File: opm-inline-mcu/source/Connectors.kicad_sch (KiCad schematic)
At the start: 32 parts, among them J1 Info, J2 VCC_IO, J3 PWMx6, J4 Fan, J6 Current Sensing, Q7 WSD90P06DN56, U2 TerminalBlock_2_P5.08mm, U3 TerminalBlock_3_P5.08mm

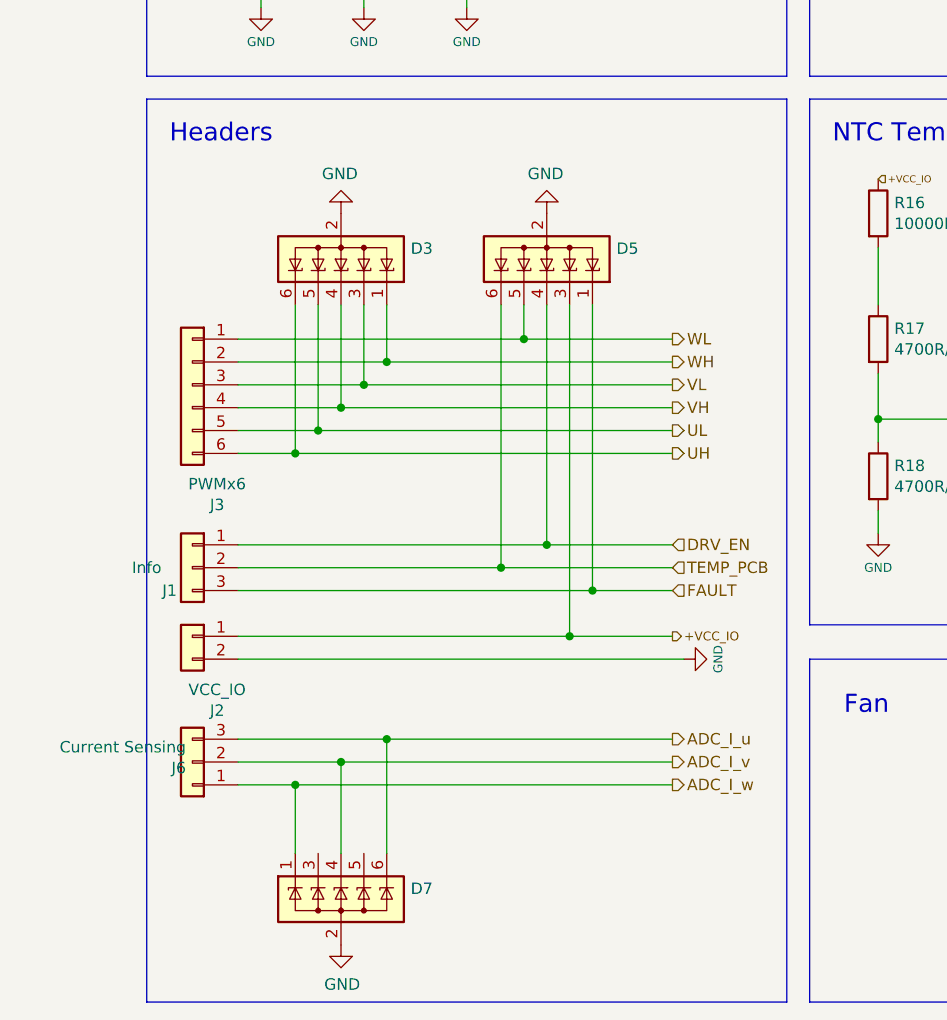
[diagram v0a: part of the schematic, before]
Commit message: update mcu
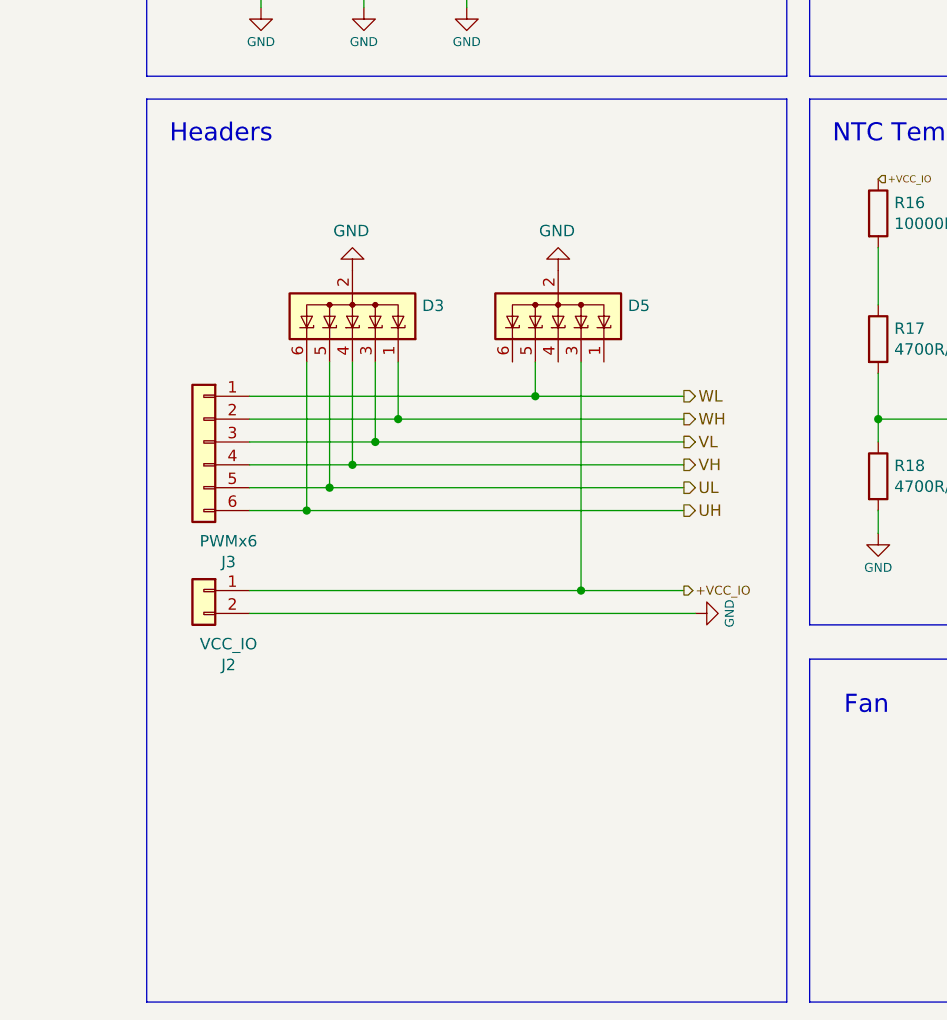
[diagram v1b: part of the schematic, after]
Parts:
- removed D7: NUP4114UCW1T2G, Libraries:NUP4114UCW1T2G, symbol Power_Protection:SP0505BAJT
- removed J1: Info, Connector_JST:JST_PH_B3B-PH-K_1x03_P2.00mm_Vertical, symbol Connector_Generic:Conn_01x03
- removed J6: Current Sensing, Connector_JST:JST_PH_B3B-PH-K_1x03_P2.00mm_Vertical, symbol Connector_Generic:Conn_01x03
- D3, D5: value NUP4114UCW1T2G -> Val**
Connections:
- net FAULT: no longer D5.1 (K)
- net TEMP_PCB: no longer D5.6 (K)
- net DRV_EN: no longer names the net of D5.4 (K)
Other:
- moved on the sheet: D3, D5, J2, J3
